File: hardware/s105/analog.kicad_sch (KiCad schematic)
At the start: 89 parts

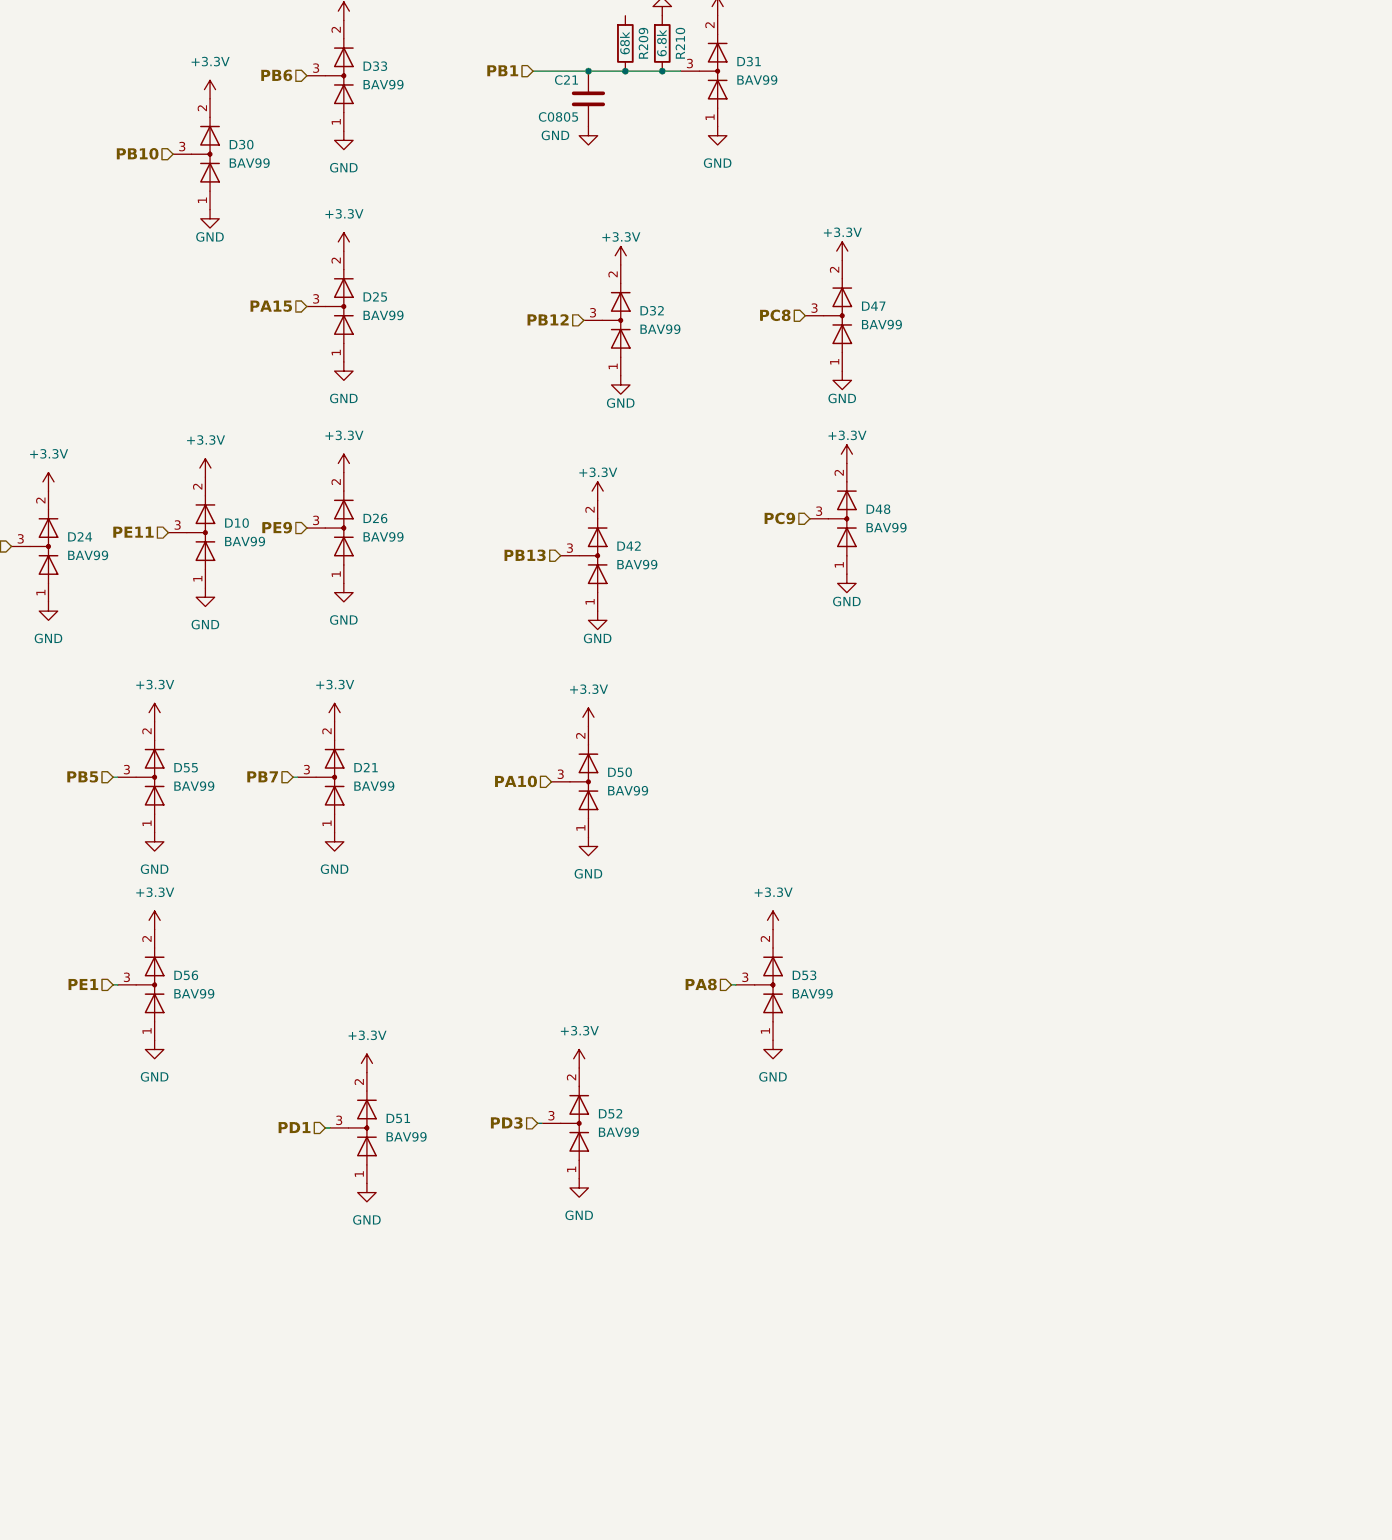
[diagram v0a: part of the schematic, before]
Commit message: can, analog inputs
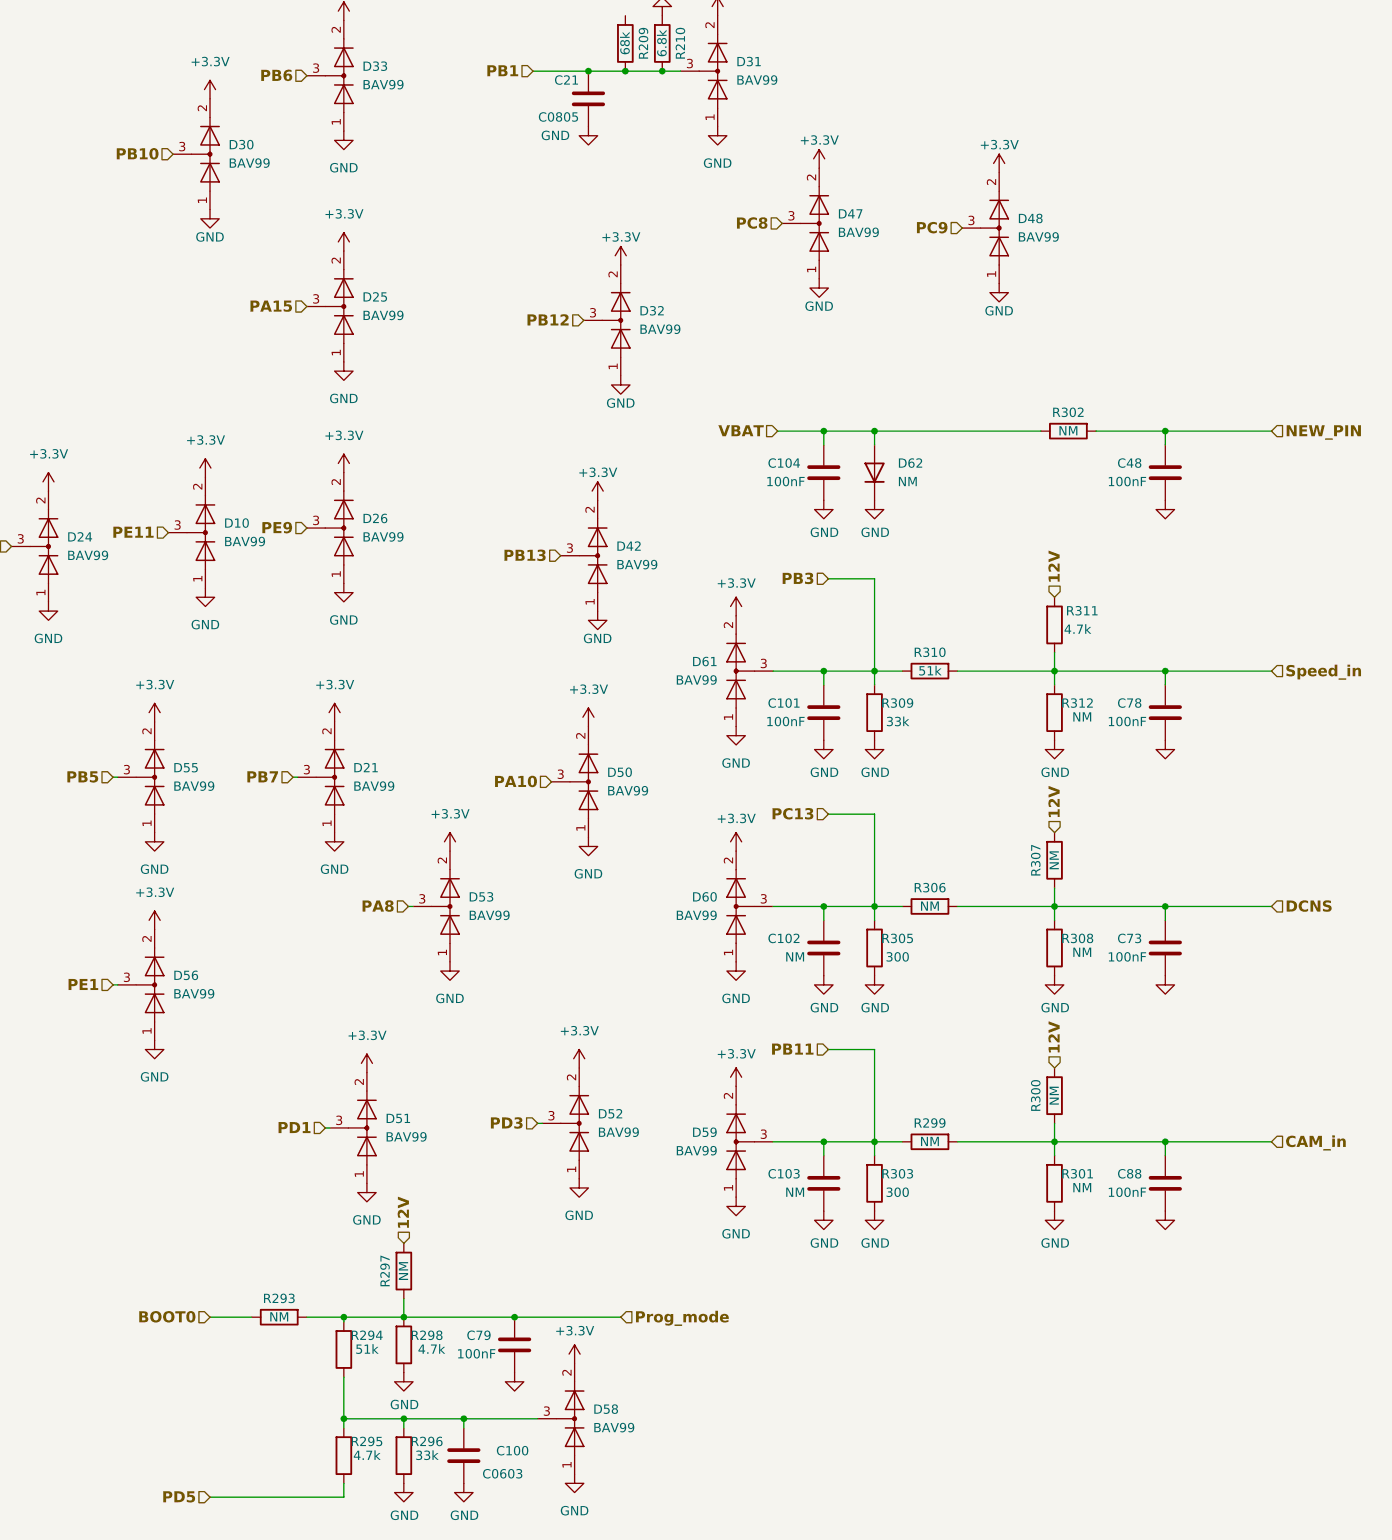
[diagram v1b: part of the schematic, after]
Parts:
- added C100: C0603, Capacitor_SMD:C_0603_1608Metric, symbol Device:C
- added C101, C104, C48, C73, C78, C79, C88: 100nF, Capacitor_SMD:C_0603_1608Metric, symbol Device:C
- added C102, C103: NM, Capacitor_SMD:C_0603_1608Metric, symbol Device:C
- added D58, D59, D60, D61: BAV99, Package_TO_SOT_SMD:SOT-23, symbol Diode:BAV99
- added D62: NM, Diode_SMD:D_SOD-123, symbol Diode:1N4148W
- added R293, R299, R306: NM, Resistor_SMD:R_0603_1608Metric, symbol Device:R
- added R294, R310: 51k, Resistor_SMD:R_0603_1608Metric, symbol Device:R
- added R295: 4.7k, Resistor_SMD:R_0603_1608Metric, symbol Device:R
- added R296, R309: 33k, Resistor_SMD:R_0603_1608Metric, symbol Device:R
- added R297, R300, R301, R302, R307, R308, R312: NM, Resistor_SMD:R_1206_3216Metric, symbol Device:R
- added R298, R311: 4.7k, Resistor_SMD:R_1206_3216Metric, symbol Device:R
- added R303, R305: 300, Resistor_SMD:R_0603_1608Metric, symbol Device:R
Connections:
- net +3.3V: now also D58.2 (A), D59.2 (A), D60.2 (A), D61.2 (A)
- net GND: now also C100.2, C101.1, C102.1, C103.1, C104.1, C48.1, C73.1, C78.1, C79.1, C88.1, D58.1 (K), D59.1 (K), D60.1 (K), D61.1 (K), D62.1 (K), R296.1, R298.1, R301.1, R303.1, R305.1, R308.1, R309.1, R312.1
- new net: C100.1, D58.3 (K), R294.1, R295.2, R296.2
- new net 12V: R297.2, R300.2, R307.2, R311.2
- new net BOOT0: R293.1
- new net CAM_in: C88.2, R299.2, R300.1, R301.2
- new net DCNS: C73.2, R306.2, R307.1, R308.2
- new net NEW_PIN: C48.2, R302.2
- new net PB11: C103.2, D59.3 (K), R299.1, R303.2
- new net PB3: C101.2, D61.3 (K), R309.2, R310.1
- new net PC13: C102.2, D60.3 (K), R305.2, R306.1
- new net PD5: R295.1
- new net Prog_mode: C79.2, R293.2, R294.2, R297.1, R298.2
- new net Speed_in: C78.2, R310.2, R311.1, R312.2
- new net VBAT: C104.2, D62.2 (A), R302.1
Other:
- moved on the sheet: D47, D48, D53

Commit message: закончила пока что
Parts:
- removed D30, D50: BAV99, Package_TO_SOT_SMD:SOT-23, symbol Diode:BAV99
- added C113, C114, C115, C116, C117, C80, C81, C82, C83: 100nF, Capacitor_SMD:C_0603_1608Metric, symbol Device:C
- added D68, D69, D70, D71: BAV99, Package_TO_SOT_SMD:SOT-23, symbol Diode:BAV99
- added R318, R322, R324: 33k, Resistor_SMD:R_0603_1608Metric, symbol Device:R
- added R319, R325, R327: 51k, Resistor_SMD:R_0603_1608Metric, symbol Device:R
- added R320, R329, R332: 4.7k, Resistor_SMD:R_1206_3216Metric, symbol Device:R
- added R321, R328, R330, R331, R333: NM, Resistor_SMD:R_1206_3216Metric, symbol Device:R
- added R323: 300, Resistor_SMD:R_0603_1608Metric, symbol Device:R
- added R326: NM, Resistor_SMD:R_0603_1608Metric, symbol Device:R
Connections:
- net +3.3V: now also D68.2 (A), D69.2 (A), D70.2 (A), D71.2 (A)
- net 12V: now also R320.2, R328.2, R330.2, R332.2
- net GND: now also R209.2, C113.1, C114.1, C115.1, C116.1, C117.1, C80.1, C81.1, C82.1, C83.1, D68.1 (K), D69.1 (K), D70.1 (K), D71.1 (K), R318.1, R321.1, R322.1, R323.1, R324.1, R329.1, R331.1, R333.1
- net PA3: now also C36.2, D38.3 (K), R214.2; no longer C35.2, D37.3 (K), R164.2
- net PC0: now also C117.2
- net PC4: now also C35.2, D37.3 (K), R164.2; no longer C36.2, D38.3 (K), R214.2
- new net DIN1: C80.2, R319.2, R320.1, R321.2
- new net DIN5: C83.2, R327.2, R332.1, R333.2
- new net DPH2: C81.2, R326.2, R330.1, R331.2
- new net PC10: C116.2, D71.3 (K), R324.2, R327.1
- new net PC11: C115.2, D70.3 (K), R323.2, R326.1
- new net PC12: C113.2, D68.3 (K), R318.2, R319.1
- new net PD4: C114.2, D69.3 (K), R322.2, R325.1
- new net Start_req: C82.2, R325.2, R328.1, R329.2
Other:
- note added: "Это все к модулям OD"
- moved on the sheet: C100, C101, C102, C103, C104, C21, C34, C35, C36, C37, C38, C48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
